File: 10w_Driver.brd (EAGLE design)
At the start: 47 x 47 mm, 35 parts, among them IC1 78L05Z, IC2 WS2811-SOP8, T1 2N3904, T2 2N3904, T3 2N3904, U1 PT4115PT4115B89E, U2 PT4115PT4115B89E, U3 PT4115PT4115B89E, X1 22-23-2031, X2 22-23-2031, X3 LED-PAD, X4 LED-PAD, X5 LED-PAD, X6 LED-PAD, X7 LED-PAD, X8 LED-PAD

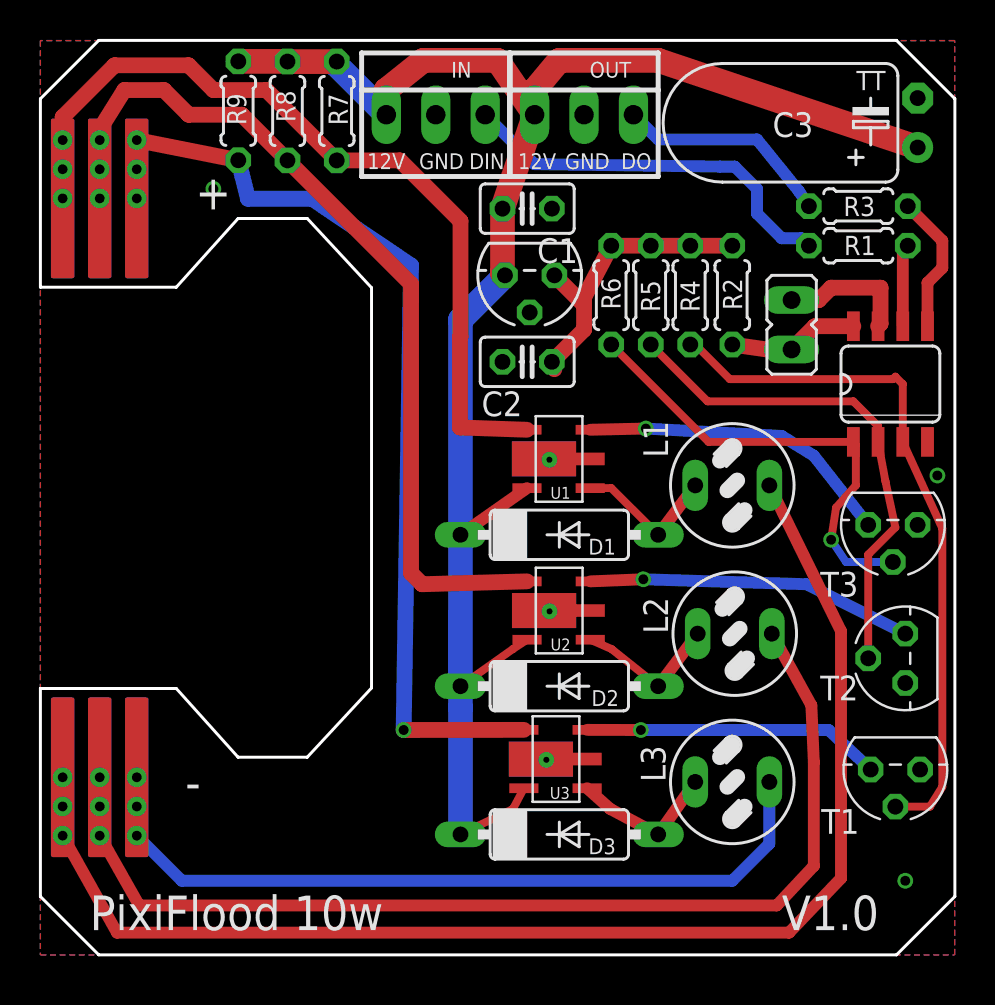
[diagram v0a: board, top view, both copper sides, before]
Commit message: Reworked Layout
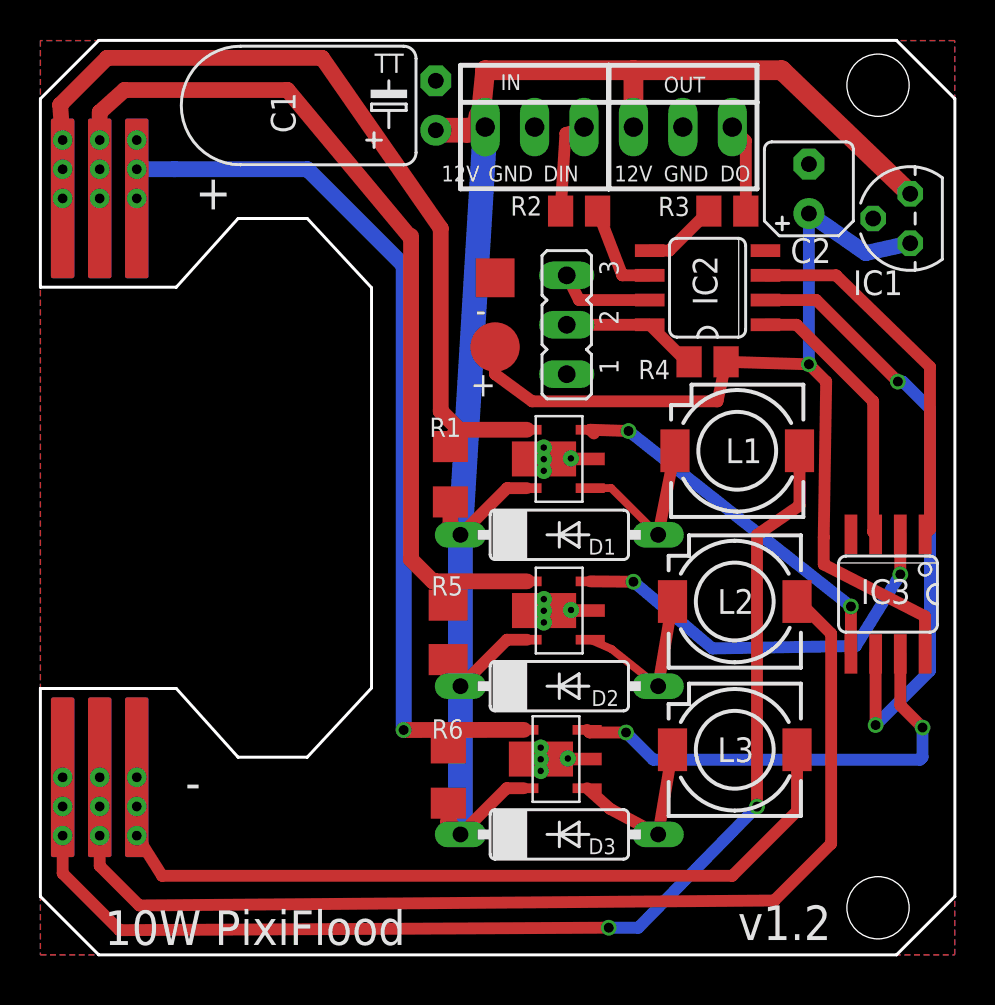
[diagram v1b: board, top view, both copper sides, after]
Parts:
- removed C3: EL 100uF, rcl:TT2D6L
- removed R7, R8, R9: .33Ohm .25w, resistor:0204/5
- removed T1, T2, T3: 2N3904, transistor:TO92
- added IC3: TC7W04FTC7W04F, MyLibrary:SO08
- added TP1: TPB2,54, testpad:B2,54
- added TP2: PTR1TP20SQ, testpad:TP20SQ
- C1: value .33uF -> EL 100uF; device rcl:C025-025X050 -> rcl:TT2D6L
- C2: device rcl:C025-025X050 -> resistor:B45181A
- JP1: device jumper:JP1 -> jumper:JP2
- L1, L2, L3: value 82114R -> SLF7045; device inductors:82114R -> inductors:SLF7045
- R1: value 33R -> .3ohm .25w; device rcl:0204/5 -> resistor:R1206
- R2: value 100ohm -> 33R; device rcl:0204/5 -> rcl:M0805
- R3: device rcl:0204/5 -> rcl:M0805
- R4: value (none) -> 100ohm; device resistor:0204/5 -> rcl:M0805
- R5: value (none) -> .3hm .25w; device resistor:0204/5 -> resistor:M1206
- R6: value (none) -> .3ohm .25w; device resistor:0204/5 -> resistor:R1206
- U1, U2, U3: device MyLibrary:SOT89-5 -> IC:SOT89-5
- X2: value 22-23-2031 -> LED-PAD; device MyLibrary:22-23-2031 -> MyLibrary:LED-PAD
- X4: value LED-PAD -> 22-23-2031; device MyLibrary:LED-PAD -> MyLibrary:22-23-2031
- moved X4 47.3 mm to (33.0, 42.5), turned to 0 degrees
- moved X3 32.8 mm to (1.14, 7.62), turned to 180 degrees
- moved X2 26.9 mm to (1.14, 40.4)
- moved R6 26.1 mm to (21.0, 9.22)
- moved R1 24.0 mm to (21.1, 24.7), turned to 270 degrees
- moved R5 20.2 mm to (21.0, 16.6)
- moved IC1 19.8 mm to (44.7, 37.8), turned to 90 degrees
- moved C2 17.0 mm to (39.5, 39.4), turned to 90 degrees
- moved JP1 11.6 mm to (27.1, 32.4), turned to 90 degrees
- moved IC2 10.6 mm to (34.3, 34.3), turned to 90 degrees
- moved R2 8.98 mm to (27.7, 38.2), turned to 0 degrees
- moved C1 7.08 mm to (20.3, 43.7), turned to 90 degrees
- moved R3 6.74 mm to (35.3, 38.2), turned to 180 degrees
- moved X1 5.12 mm to (25.4, 42.5)
- moved R4 3.54 mm to (34.3, 30.5), turned to 180 degrees
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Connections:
- removed net N$20: IC2.1, R6.2, T3.2
- new net N$19: IC2.2, IC3.6
- net +12V: now also C1.+, R1.2, R5.2, R6.2, X4.1; no longer C1.1, C3.+, R7.1, R8.1, R9.1, X2.1
- net +5V: now also C2.+, IC3.8, TP1.TP; no longer C2.1, R2.1, R5.1, R6.1
- net BLUE: now also IC3.7; no longer T1.1
- net BOUT: now also R6.1; no longer R9.2
- net GND: now also C1.-, C2.-, IC3.4, TP2.TP, U1.2A@3, U1.2A@4, U2.2A@3, U2.2A@4, U3.2A@3, U3.2A@4, X4.2; no longer C1.2, C2.2, C3.-, T1.3, T2.3, T3.3, X2.2
- net GOUT: now also R5.1; no longer R8.2
- net GREEN: now also IC3.2; no longer T2.1
- net N$14: now also JP1.2, R4.2; no longer JP1.1, R2.2
- net N$15: now also IC2.1, IC3.3; no longer IC2.3, R4.2, T1.2
- net N$16: now also IC2.3, IC3.1; no longer IC2.7, JP1.2
- net N$18: now also IC2.7, JP1.3; no longer IC2.2, R5.2, T2.2
- net N$3: now also X3.P$1@1, X3.P$1@2, X3.P$1@3; no longer X4.P$1@1, X4.P$1@2, X4.P$1@3
- net N$4: now also X4.3; no longer X2.3
- net N$6: now also R2.1; no longer R1.1
- net N$8: now also R2.2; no longer R1.2
- net RED: now also IC3.5; no longer T3.1
- net ROUT: now also R1.1, X2.P$1@1, X2.P$1@2, X2.P$1@3; no longer R7.2, X3.P$1@1, X3.P$1@2, X3.P$1@3
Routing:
- net +5V: track 15.8 -> 51.7 mm, vias 0 -> 1
- net N$19: track 0.00 -> 31.8 mm, vias 0 -> 2
- net N$20: track 23.8 -> 0.00 mm, vias 1 -> 0
- net N$15: track 36.0 -> 14.1 mm
- net N$18: track 26.0 -> 5.05 mm
- net N$6: track 20.1 -> 5.02 mm
- net N$16: track 6.87 -> 19.1 mm
- net BLUE: track 15.4 -> 23.7 mm, vias 1 -> 2
- net N$4: track 11.2 -> 4.61 mm
- net +12V: track 93.0 -> 87.5 mm
- net N$10: track 37.4 -> 42.6 mm
- net GREEN: track 16.8 -> 21.3 mm, vias 1 -> 2
- net N$3: track 68.2 -> 63.9 mm, vias 0 -> 2
- net N$7: track 7.22 -> 3.88 mm
- net GOUT: track 45.9 -> 49.0 mm
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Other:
- board text added: "10W PixiFlood"
- board text added: "AJ Reynolds"
- board text added: "stampedeboss@gmail.com"
- board text added: "v1.2"
- board text removed: "PixiFlood 10w"
- board text removed: "V1.0"
